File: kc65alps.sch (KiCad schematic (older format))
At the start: 14 parts

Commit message: Schematic update
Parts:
- removed SW?: SW_Push, symbol Switch:SW_Push
- added J?: AVR-ISP-6, symbol Connector:AVR-ISP-6
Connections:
- net labels added: MISO, MOSI, RST, SCK
- wire segments 41 -> 48
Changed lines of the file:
@@
 EESchema Schematic File Version 4
+LIBS:kc65alps-cache
 EELAYER 30 0
 EELAYER END
@@
 	1250 2150 1250 2250
 $Comp
-L Switch:SW_Push SW?
-U 1 1 5DF9B2B6
-P 1550 1500
-F 0 "SW?" H 1550 1785 50  0000 C CNN
-F 1 "SW_Push" H 1550 1694 50  0000 C CNN
-F 2 "" H 1550 1700 50  0001 C CNN
-F 3 "~" H 1550 1700 50  0001 C CNN
-	1    1550 1500
-	1    0    0    -1
-$EndComp
-$Comp
-L power:GND #PWR?
-U 1 1 5DF9C33C
-P 1200 1500
-F 0 "#PWR?" H 1200 1250 50  0001 C CNN
-F 1 "GND" H 1205 1327 50  0000 C CNN
-F 2 "" H 1200 1500 50  0001 C CNN
-F 3 "" H 1200 1500 50  0001 C CNN
-	1    1200 1500
-	1    0    0    -1
-$EndComp
-Wire Wire Line
-	1200 1500 1350 1500
-Wire Wire Line
-	1750 1500 1750 1600
-Wire Wire Line
-	1750 1600 1800 1600
-$Comp
 L Device:R_Small R?
 U 1 1 5DF9EA48
@@
 Text GLabel 650  2700 0    50   Input ~ 0
 D-
+$Comp
+L Connector:AVR-ISP-6 J?
+U 1 1 5DF707AD
+P 4600 1750
+F 0 "J?" H 4321 1846 50  0000 R CNN
+F 1 "AVR-ISP-6" H 4321 1755 50  0000 R CNN
+F 2 "" V 4350 1800 50  0001 C CNN
+F 3 " ~" H 3325 1200 50  0001 C CNN
+	1    4600 1750
+	1    0    0    -1
+$EndComp
+$Comp
+L power:+5V #PWR?
+U 1 1 5DF73003
+P 4500 1100
+F 0 "#PWR?" H 4500 950 50  0001 C CNN
+F 1 "+5V" H 4515 1273 50  0000 C CNN
+F 2 "" H 4500 1100 50  0001 C CNN
+F 3 "" H 4500 1100 50  0001 C CNN
+	1    4500 1100
+	1    0    0    -1
+$EndComp
+$Comp
+L power:GND #PWR?
+U 1 1 5DF73F7A
+P 4500 2300
+F 0 "#PWR?" H 4500 2050 50  0001 C CNN
+F 1 "GND" H 4505 2127 50  0000 C CNN
+F 2 "" H 4500 2300 50  0001 C CNN
+F 3 "" H 4500 2300 50  0001 C CNN
+	1    4500 2300
+	1    0    0    -1
+$EndComp
+Text GLabel 5200 1550 2    50   Input ~ 0
+MISO
+Text GLabel 5200 1650 2    50   Input ~ 0
+MOSI
+Text GLabel 5250 1750 2    50   Input ~ 0
+SCK
+Text GLabel 5250 1850 2    50   Input ~ 0
+RST
+Wire Wire Line
+	5000 1550 5200 1550
+Wire Wire Line
+	5200 1650 5000 1650
+Wire Wire Line
+	5000 1750 5250 1750
+Wire Wire Line
+	5250 1850 5000 1850
+Wire Wire Line
+	4500 1250 4500 1100
+Wire Wire Line
+	4500 2150 4500 2300
+Text GLabel 1550 1600 0    50   Input ~ 0
+RST
+Wire Wire Line
+	1550 1600 1800 1600
+Text GLabel 3250 1900 2    50   Input ~ 0
+MISO
+Text GLabel 3250 1800 2    50   Input ~ 0
+MOSI
+Text GLabel 3250 1700 2    50   Input ~ 0
+SCK
+Wire Wire Line
+	3050 1700 3250 1700
+Wire Wire Line
+	3250 1800 3050 1800
+Wire Wire Line
+	3050 1900 3250 1900
 $EndSCHEMATC

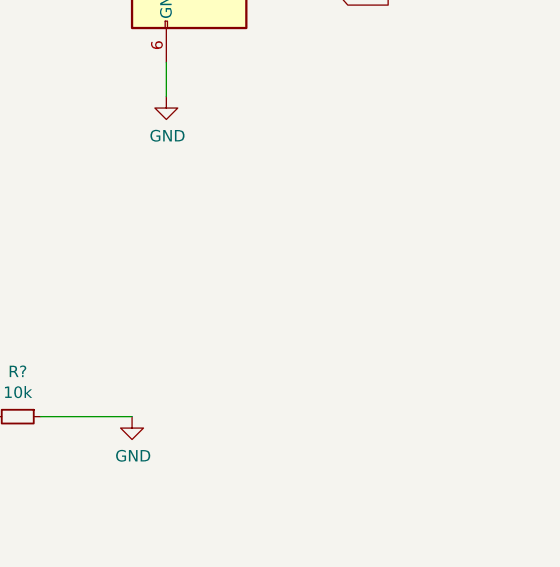
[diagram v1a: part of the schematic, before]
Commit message: Schematic Update
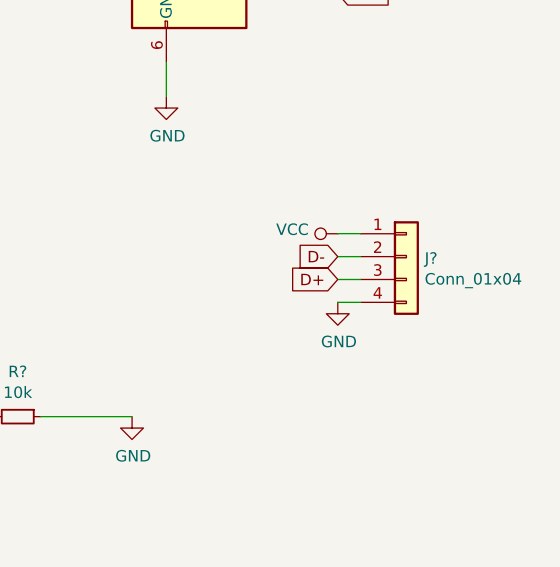
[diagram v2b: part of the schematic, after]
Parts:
- added J?: Conn_01x04, symbol Connector_Generic:Conn_01x04
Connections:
- net D+: now also J?.3 (Pin_3)
- net D-: now also J?.2 (Pin_2)
- net GND: now also J?.4 (Pin_4)
- new net VCC: J?.1 (Pin_1)
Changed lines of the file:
@@
 Wire Wire Line
 	3050 1900 3250 1900
+$Comp
+L Connector_Generic:Conn_01x04 J?
+U 1 1 5DF85843
+P 5550 3000
+F 0 "J?" H 5630 2992 50  0000 L CNN
+F 1 "Conn_01x04" H 5630 2901 50  0000 L CNN
+F 2 "" H 5550 3000 50  0001 C CNN
+F 3 "~" H 5550 3000 50  0001 C CNN
+	1    5550 3000
+	1    0    0    -1
+$EndComp
+$Comp
+L power:VCC #PWR?
+U 1 1 5DF868E4
+P 5250 2900
+F 0 "#PWR?" H 5250 2750 50  0001 C CNN
+F 1 "VCC" V 5268 3027 50  0000 L CNN
+F 2 "" H 5250 2900 50  0001 C CNN
+F 3 "" H 5250 2900 50  0001 C CNN
+	1    5250 2900
+	0    -1   -1   0
+$EndComp
+$Comp
+L power:GND #PWR?
+U 1 1 5DF87727
+P 5250 3200
+F 0 "#PWR?" H 5250 2950 50  0001 C CNN
+F 1 "GND" H 5255 3027 50  0000 C CNN
+F 2 "" H 5250 3200 50  0001 C CNN
+F 3 "" H 5250 3200 50  0001 C CNN
+	1    5250 3200
+	1    0    0    -1
+$EndComp
+Text GLabel 5250 3000 0    50   Input ~ 0
+D-
+Text GLabel 5250 3100 0    50   Input ~ 0
+D+
+Wire Wire Line
+	5250 3200 5350 3200
+Wire Wire Line
+	5250 3100 5350 3100
+Wire Wire Line
+	5250 3000 5350 3000
+Wire Wire Line
+	5250 2900 5350 2900
 $EndSCHEMATC

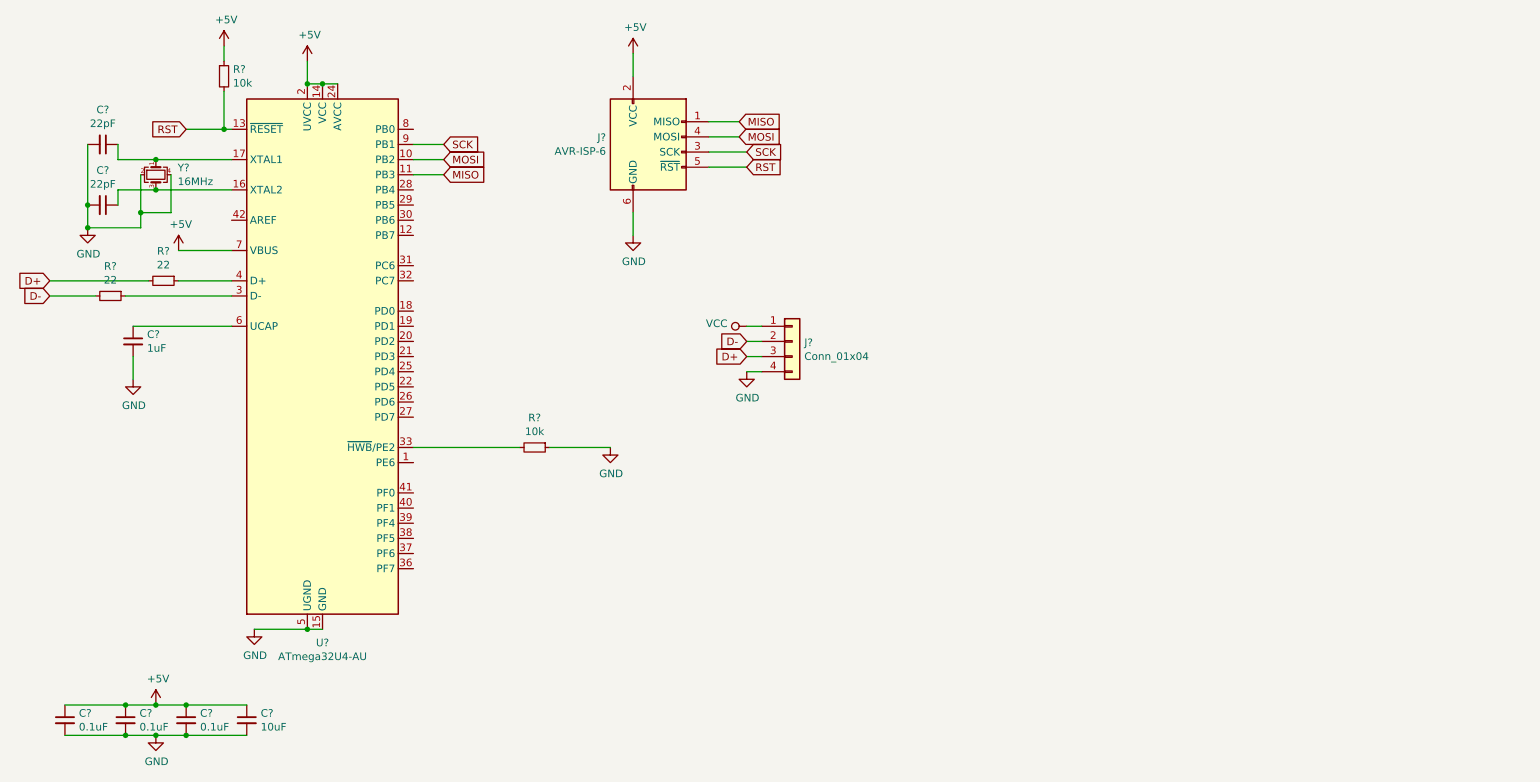
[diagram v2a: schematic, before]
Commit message: Schematic Update
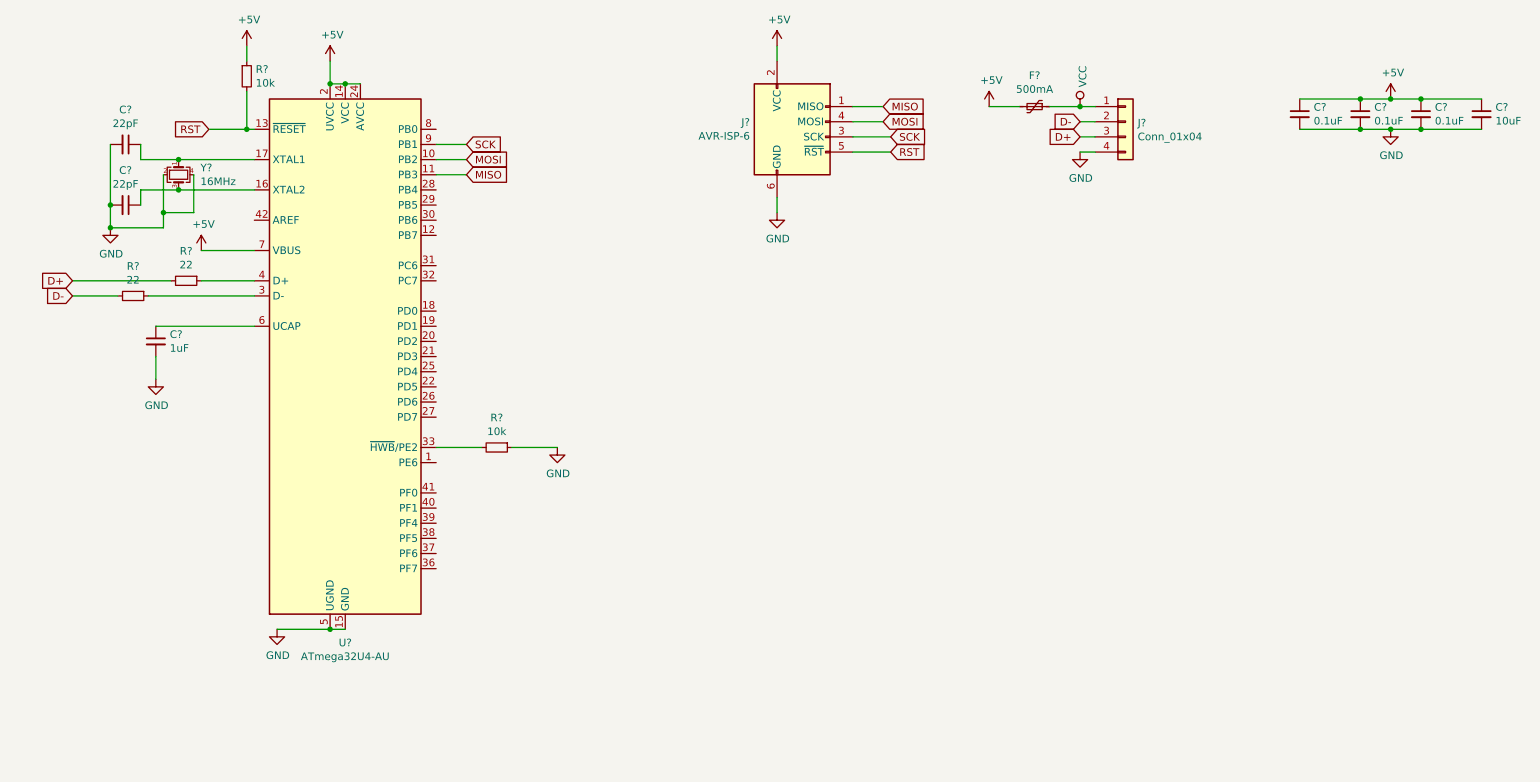
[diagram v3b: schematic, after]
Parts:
- added F?: 500mA, symbol Device:Polyfuse_Small
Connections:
- net +5V: now also F?.2
- net VCC: now also F?.1
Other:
- moved on the sheet: C?, J?, R?, U?, Y?

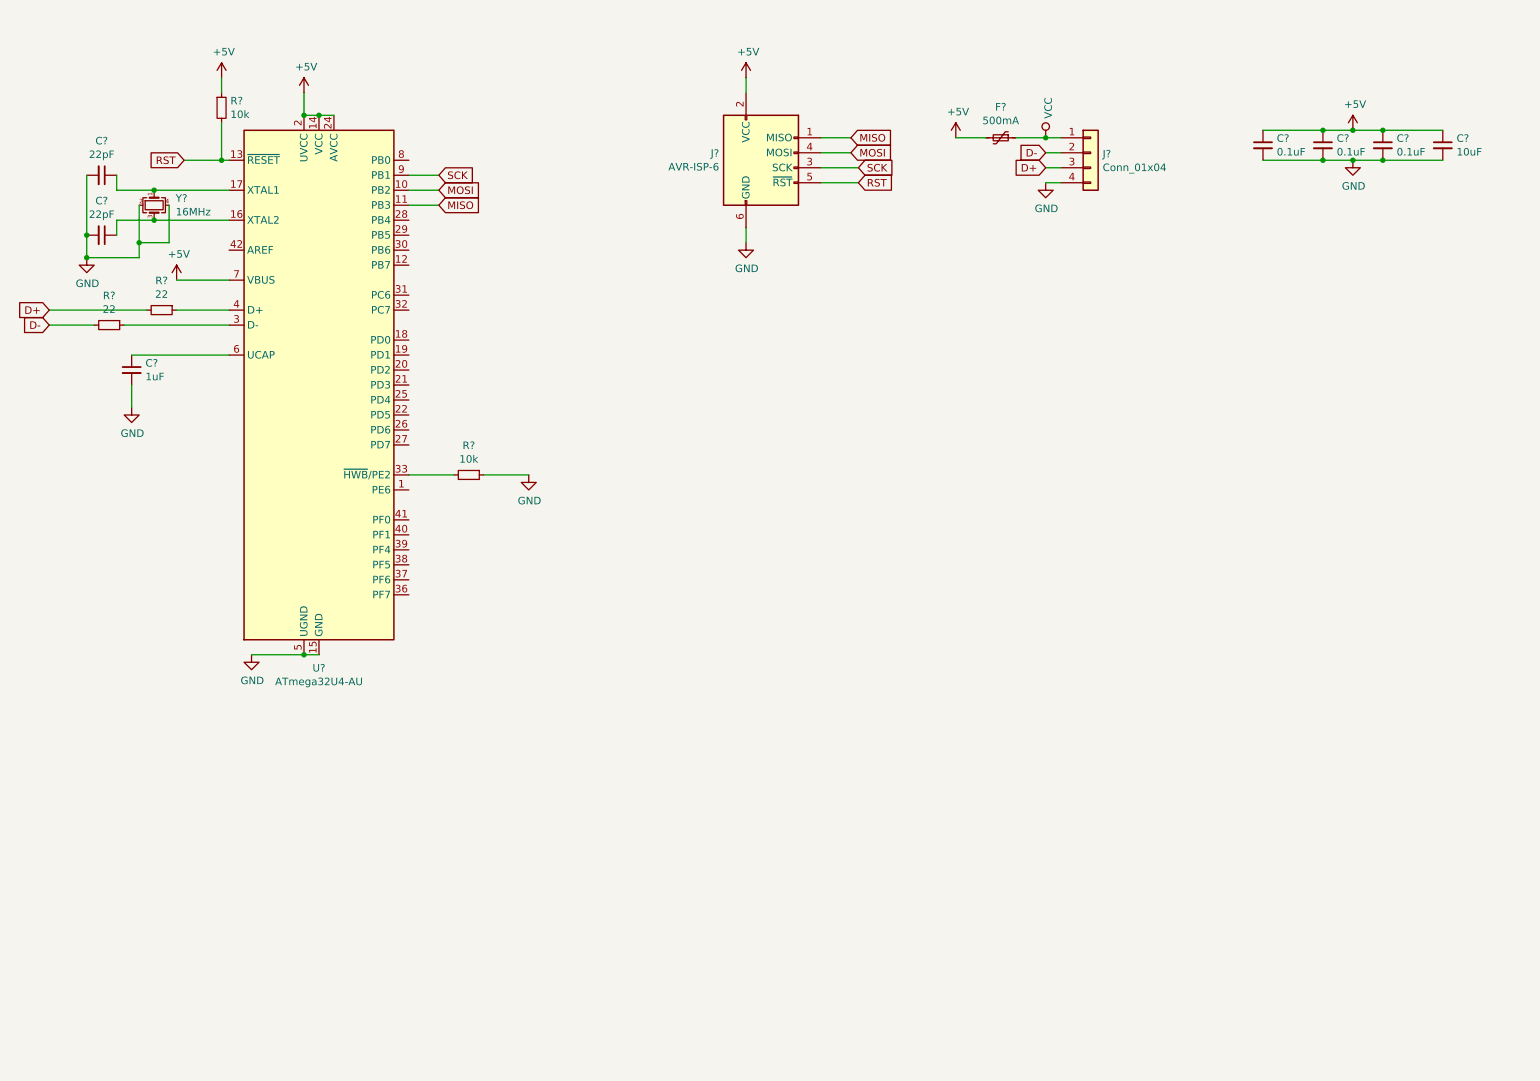
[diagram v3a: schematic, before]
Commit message: Schematic update
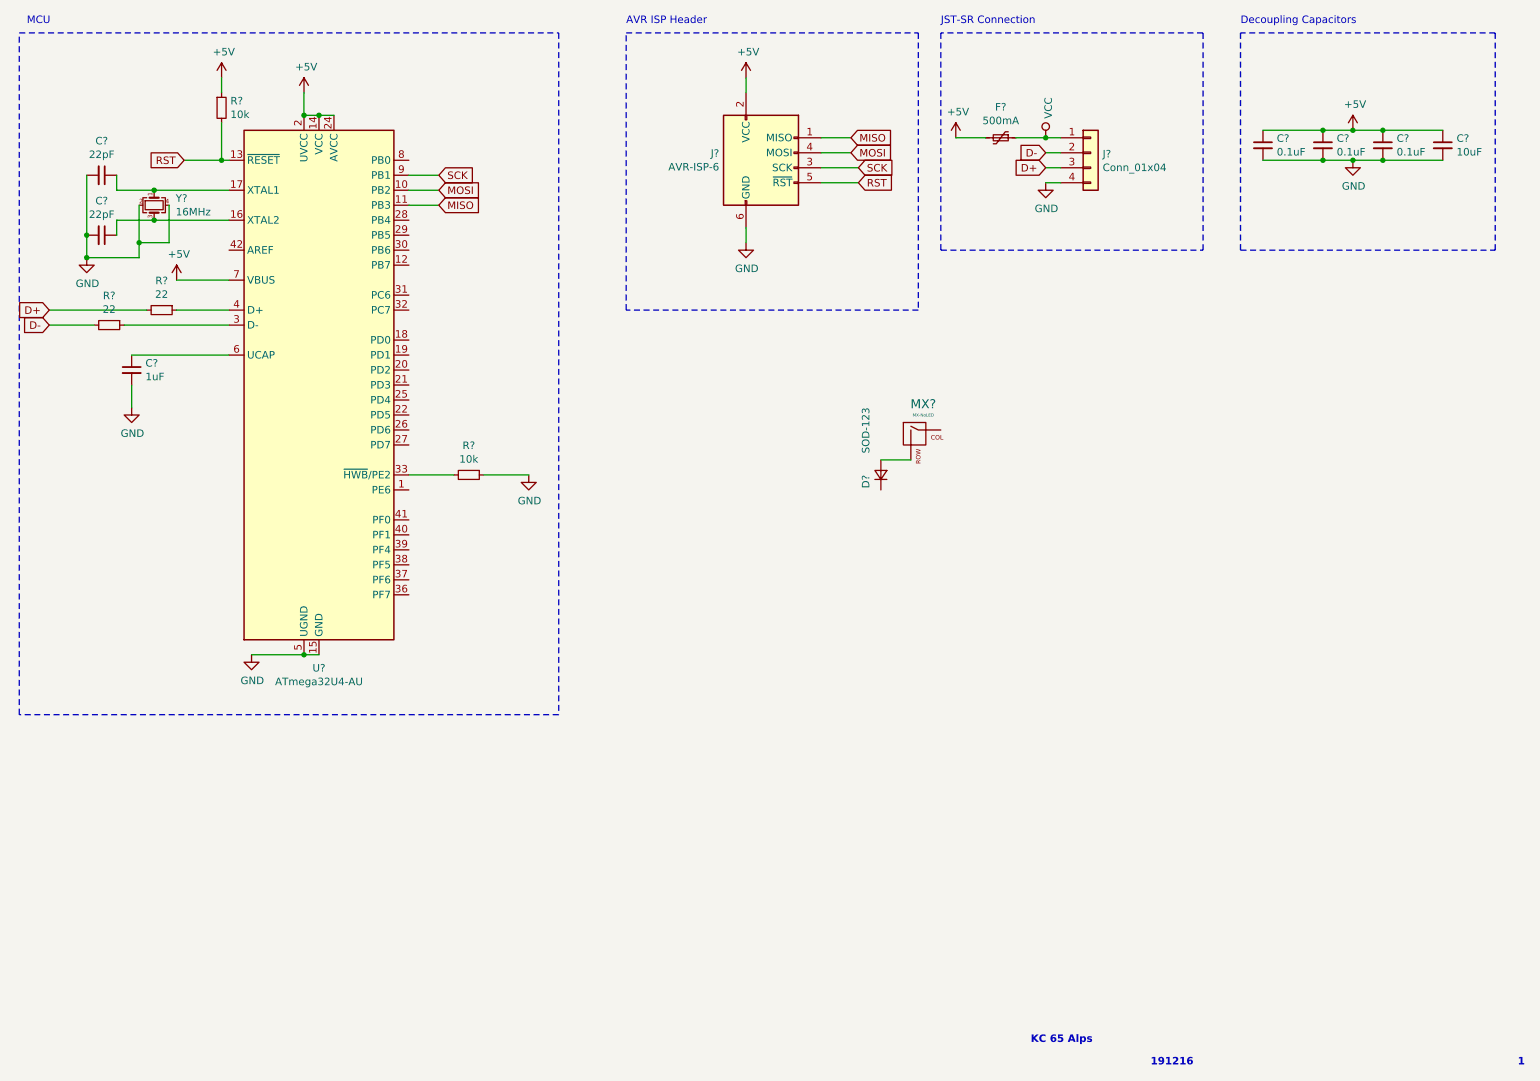
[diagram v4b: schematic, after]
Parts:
- added D?: SOD-123, symbol Device:D_Small
- added MX?: MX-NoLED, symbol MX_Alps_Hybrid:MX-NoLED
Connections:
- new net: D?.2 (A), MX?.2 (ROW)
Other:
- note added: "1"
- note added: "191216"
- note added: "AVR ISP Header"
- note added: "Decoupling Capacitors"
- note added: "JST-SR Connection"
- note added: "KC 65 Alps"
- note added: "MCU"
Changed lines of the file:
@@
 Wire Wire Line
 	3700 3700 4000 3700
+Wire Notes Line
+	600  750  4200 750
+Wire Notes Line
+	4200 750  4200 5300
+Wire Notes Line
+	4200 5300 600  5300
+Wire Notes Line
+	600  5300 600  750
+Wire Notes Line
+	4650 750  6600 750
+Wire Notes Line
+	6600 750  6600 2600
+Wire Notes Line
+	6600 2600 4650 2600
+Wire Notes Line
+	4650 2600 4650 750
+Wire Notes Line
+	6750 750  6750 2200
+Wire Notes Line
+	6750 2200 8500 2200
+Wire Notes Line
+	8500 2200 8500 750
+Wire Notes Line
+	8500 750  6750 750
+Wire Notes Line
+	8750 750  8750 2200
+Wire Notes Line
+	8750 2200 10450 2200
+Wire Notes Line
+	10450 2200 10450 750
+Wire Notes Line
+	10450 750  8750 750
+Text Notes 650  700  0    50   ~ 0
+MCU
+Text Notes 4650 700  0    50   ~ 0
+AVR ISP Header
+Text Notes 6750 700  0    50   ~ 0
+JST-SR Connection
+Text Notes 8750 700  0    50   ~ 0
+Decoupling Capacitors
+Text Notes 7350 7500 0    50   ~ 10
+KC 65 Alps
+Text Notes 8150 7650 0    50   ~ 10
+191216
+Text Notes 10600 7650 0    50   ~ 10
+1
+$Comp
+L MX_Alps_Hybrid:MX-NoLED MX?
+U 1 1 5DF931BD
+P 6600 3450
+F 0 "MX?" H 6633 3673 60  0000 C CNN
+F 1 "MX-NoLED" H 6633 3599 20  0000 C CNN
+F 2 "" H 5975 3425 60  0001 C CNN
+F 3 "" H 5975 3425 60  0001 C CNN
+	1    6600 3450
+	1    0    0    -1
+$EndComp
+$Comp
+L Device:D_Small D?
+U 1 1 5DF95296
+P 6350 3700
+F 0 "D?" H 6350 3800 50  0000 R CNN
+F 1 "SOD-123" H 6800 3800 50  0000 R CNN
+F 2 "" V 6350 3700 50  0001 C CNN
+F 3 "~" V 6350 3700 50  0001 C CNN
+	1    6350 3700
+	0    -1   -1   0
+$EndComp
+Wire Wire Line
+	6350 3600 6550 3600
 $EndSCHEMATC
